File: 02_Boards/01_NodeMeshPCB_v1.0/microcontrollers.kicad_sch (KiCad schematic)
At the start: 19 parts, among them U11 nRF52840, U8 ESP32-C6-MINI-1U-H4, Y1 32NHz, Y2 32768kHz

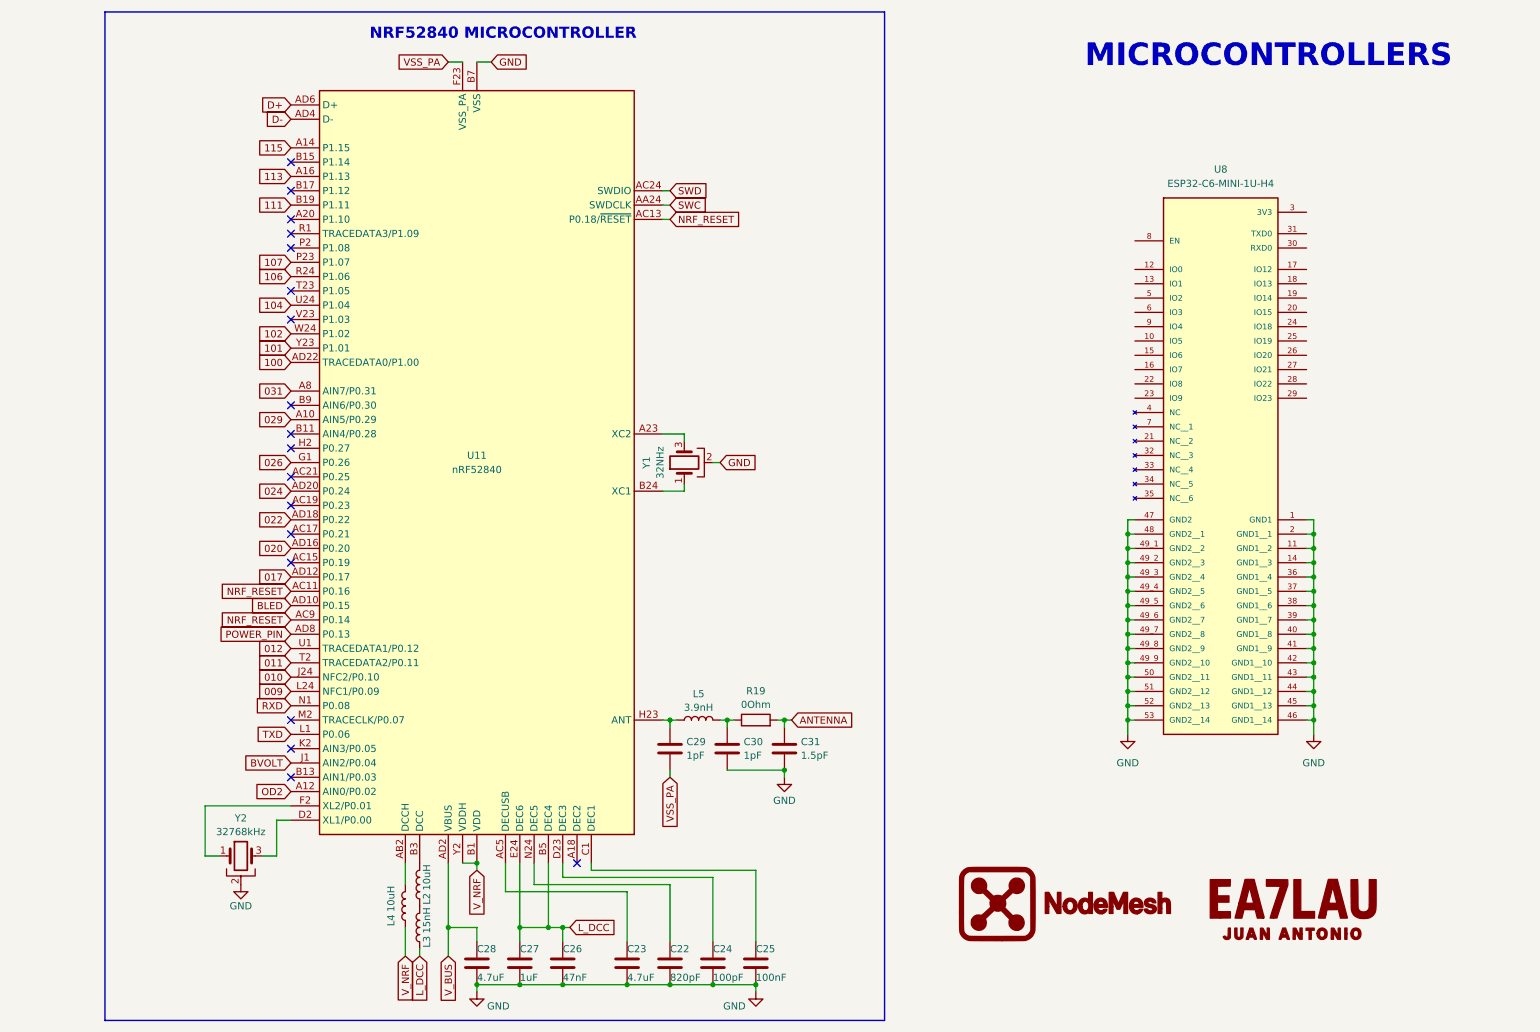
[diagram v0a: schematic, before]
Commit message: PCB placement
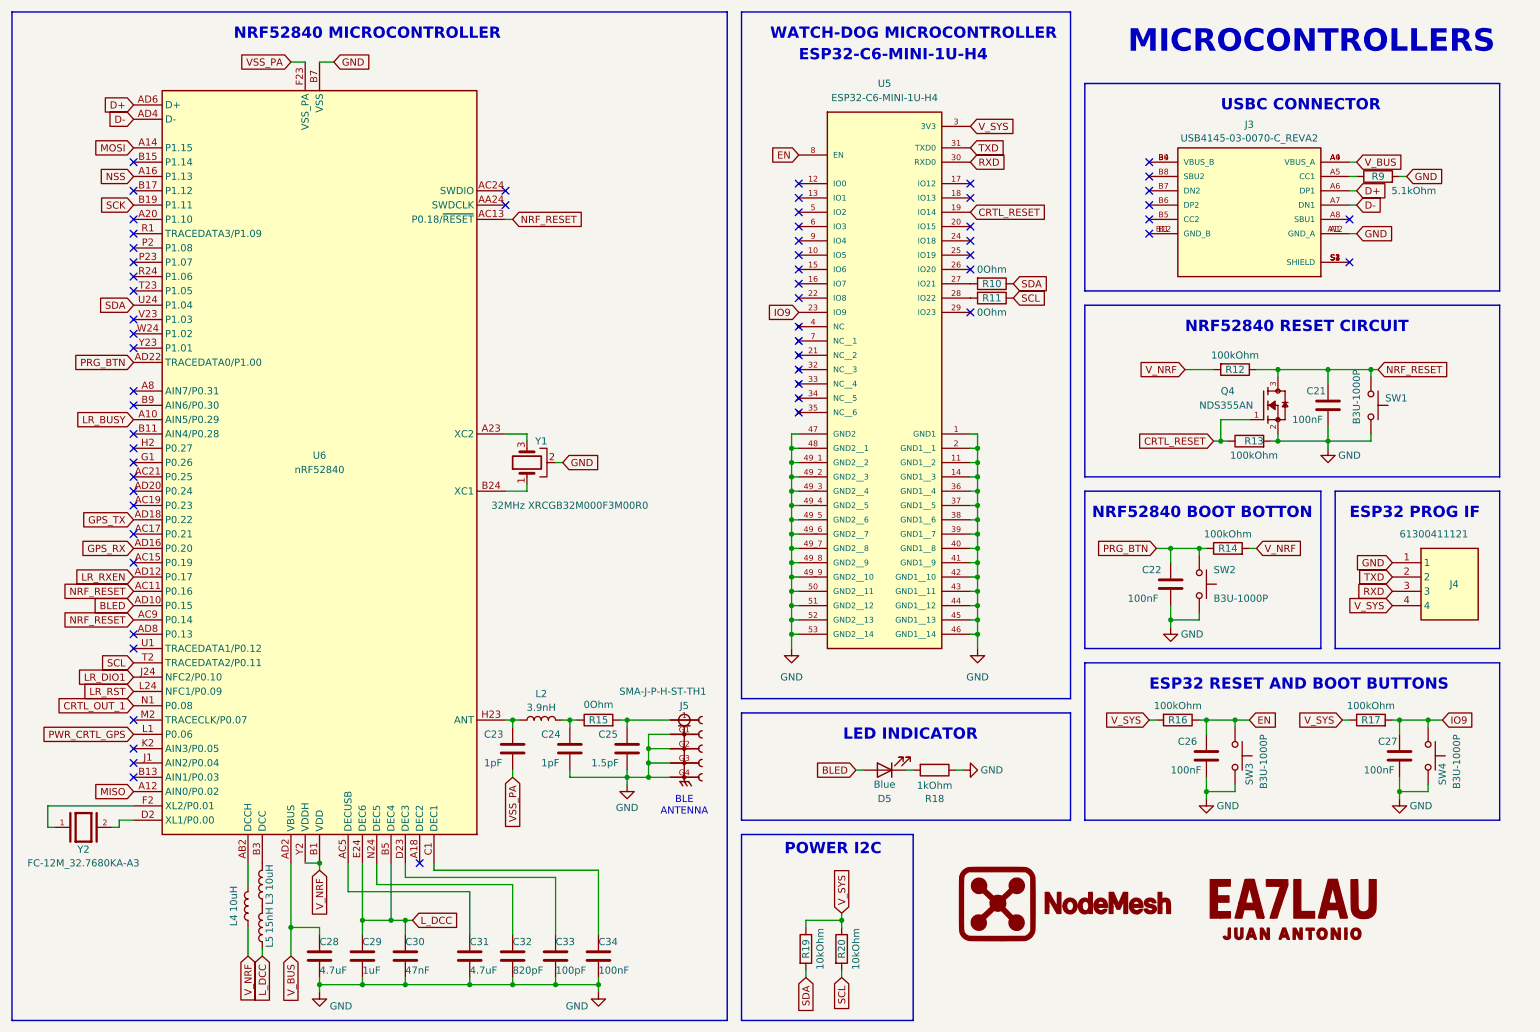
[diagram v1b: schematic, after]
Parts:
- removed Y2: 32768kHz, symbol Device:Crystal_GND2
- added C21, C22, C26, C27: 100nF, Capacitor_SMD:C_0603_1608Metric, symbol Device:C
- added D5: Blue, LED_SMD:LED_0603_1608Metric, symbol Device:LED
- added J3: USB4145-03-0070-C_REVA2, 01_Footprints:USB4145-03-0070-C, symbol USB4145-03-0070-C:USB4145-03-0070-C_REVA2
- added J4: 61300411121, 01_Footprints:61300411121, symbol 61300411121:61300411121
- added J5: SMA-J-P-H-ST-TH1, 01_Footprints:SMA-J-P-H-ST-TH1, symbol SMA-J-P-H-ST-TH1:SMA-J-P-H-ST-TH1
- added Q4: NDS355AN, 01_Footprints:NDS355AN, symbol NDS355AN:NDS355AN
- added R10, R11: 0Ohm, Resistor_SMD:R_0603_1608Metric, symbol Device:R
- added R12, R13, R14, R16, R17: 100kOhm, Resistor_SMD:R_0603_1608Metric, symbol Device:R
- added R18: 1kOhm, Resistor_SMD:R_0603_1608Metric, symbol Device:R
- added R19, R20: 10kOhm, Resistor_SMD:R_0603_1608Metric, symbol Device:R
- added R9: 5.1kOhm, Resistor_SMD:R_0603_1608Metric, symbol Device:R
- added SW1, SW2, SW3, SW4: B3U-1000P, Button_Switch_SMD:SW_SPST_B3U-1000P, symbol Switch:SW_Push
- added Y2: FC-12M_32.7680KA-A3, 01_Footprints:FC-12M_327680KA-A3, symbol FC-12M_327680KA-A3:FC-12M_32.7680KA-A3
- C23: renamed from C29; footprint (none) -> Capacitor_SMD:C_0603_1608Metric
- C24: renamed from C30; footprint (none) -> Capacitor_SMD:C_0603_1608Metric
- C25: renamed from C31; footprint (none) -> Capacitor_SMD:C_0603_1608Metric
- C28: footprint (none) -> Capacitor_SMD:C_0603_1608Metric
- C29: renamed from C27; footprint (none) -> Capacitor_SMD:C_0603_1608Metric
- C30: renamed from C26; footprint (none) -> Capacitor_SMD:C_0603_1608Metric
- C31: renamed from C23; footprint (none) -> Capacitor_SMD:C_0603_1608Metric
- C32: renamed from C22; footprint (none) -> Capacitor_SMD:C_0603_1608Metric
- C33: renamed from C24; footprint (none) -> Capacitor_SMD:C_0603_1608Metric
- C34: renamed from C25; footprint (none) -> Capacitor_SMD:C_0603_1608Metric
- L2: renamed from L5; footprint (none) -> Inductor_SMD:L_0603_1608Metric
- L3: renamed from L2; footprint (none) -> Inductor_SMD:L_0603_1608Metric
- L4: footprint (none) -> Inductor_SMD:L_0603_1608Metric
- L5: renamed from L3; footprint (none) -> Inductor_SMD:L_0603_1608Metric
- R15: renamed from R19; footprint (none) -> Resistor_SMD:R_0603_1608Metric
- U5: renamed from U8; footprint ESP32-C6-MINI-1U-H4:XCVR_ESP32-C6-MINI-1U-H4 -> 01_Footprints:ESP32-C6-MINI-1U-H4
- Y1: value 32NHz -> 32MHz XRCGB32M000F3M00R0; footprint (none) -> 01_Footprints:XRCGB32M000F3M00R0
- renumbered U11 to U6
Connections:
- net BLED: now also D5.2 (A)
- net D+: now also J3.A6 (DP1)
- net D-: now also J3.A7 (DN1)
- net GND: now also C21.2, C22.2, C26.2, C27.2, J3.A1 (GND_A), J3.A12 (GND_A), J4.1, J5.G1, J5.G2, J5.G3, J5.G4, Q4.2, R13.2, R18.1, R9.2, SW1.2, SW2.2, SW3.2, SW4.2
- net NRF_RESET: now also C21.1, Q4.3, R12.1, SW1.1
- net RXD: now also U5.30 (RXD0), J4.3; no longer U6.N1 (P0.08)
- net TXD: now also U5.31 (TXD0), J4.2; no longer U6.L1 (P0.06)
- net V_BUS: now also J3.A4 (VBUS_A), J3.A9 (VBUS_A)
- net V_NRF: now also R12.2, R14.2
- net at U6.D2 (XL1/P0.00): now also Y2.2
- net at U6.F2 (XL2/P0.01): now also Y2.1
- net CRTL_RESET: now reaches U5.19 (IO14)
- net CRTL_RESET: now also Q4.1, R13.1
- net IO9: now reaches U5.23 (IO9)
- net IO9: now also C27.1, R17.2, SW4.1
- net at U5.27 (IO21): now also R10.2
- net at U5.28 (IO22): now also R11.2
- net V_SYS: now reaches U5.3 (3V3)
- net V_SYS: now also J4.4, R16.2, R17.1, R19.1, R20.1
- net EN: now reaches U5.8 (EN)
- net EN: now also C26.1, R16.1, SW3.1
- net 009 renamed LR_RST
- net 010 renamed LR_DIO1
- net 011 renamed SCL
- net SCL: now also R11.1, R20.2
- net 012: no longer names the net of U6.U1 (TRACEDATA1/P0.12)
- net 017 renamed LR_RXEN
- net 020 renamed GPS_RX
- net 022 renamed GPS_TX
- net 024: no longer names the net of U6.AD20 (P0.24)
- net 026: no longer names the net of U6.G1 (P0.26)
- net 029 renamed LR_BUSY
- net 031: no longer names the net of U6.A8 (AIN7/P0.31)
- net 100 renamed PRG_BTN
- net PRG_BTN: now also C22.1, R14.1, SW2.1
- net 101: no longer names the net of U6.Y23 (P1.01)
- net 102: no longer names the net of U6.W24 (P1.02)
- net 104 renamed SDA
- net SDA: now also R10.1, R19.2
- net 106: no longer names the net of U6.R24 (P1.06)
- net 107: no longer names the net of U6.P23 (P1.07)
- net 111 renamed SCK
- net 113 renamed NSS
- net 115 renamed MOSI
- net ANTENNA: no longer names the net of C25.1, R15.2
- net ANTENNA: now also J5.1
- net BVOLT: no longer names the net of U6.J1 (AIN2/P0.04)
- net OD2 renamed MISO
- net POWER_PIN: no longer names the net of U6.AD8 (P0.13)
- net SWC: no longer names the net of U6.AA24 (SWDCLK)
- net SWD: no longer names the net of U6.AC24 (SWDIO)
- new net: J3.A5 (CC1), R9.1
- new net: J3.B1 (GND_B), J3.B12 (GND_B)
- new net: J3.B4 (VBUS_B), J3.B9 (VBUS_B)
- new net: J3.S1 (SHIELD), J3.S2 (SHIELD), J3.S3 (SHIELD), J3.S4 (SHIELD)
- new net: D5.1 (K), R18.2
- new net CRTL_OUT_1: U6.N1 (P0.08)
- new net PWR_CRTL_GPS: U6.L1 (P0.06)
- no-connect marks 18 -> 61
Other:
- note added: "BLE ANTENNA"
- note added: "ESP32 PROG IF"
- note added: "ESP32 RESET AND BOOT BUTTONS"
- note added: "ESP32-C6-MINI-1U-H4"
- note added: "LED INDICATOR"
- note added: "NRF52840 BOOT BOTTON"
- note added: "NRF52840 RESET CIRCUIT"
- note added: "POWER I2C"
- note added: "USBC CONNECTOR"
- note added: "WATCH-DOG MICROCONTROLLER"
- moved on the sheet: C23, C24, C25, C28, C29, C30, C31, C32, C33, C34, L2, L3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
